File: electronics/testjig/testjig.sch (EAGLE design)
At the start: 13 parts, among them J3 ISP/DUT, Q1 12MHz, U1 MCP1824, U2 TINY84

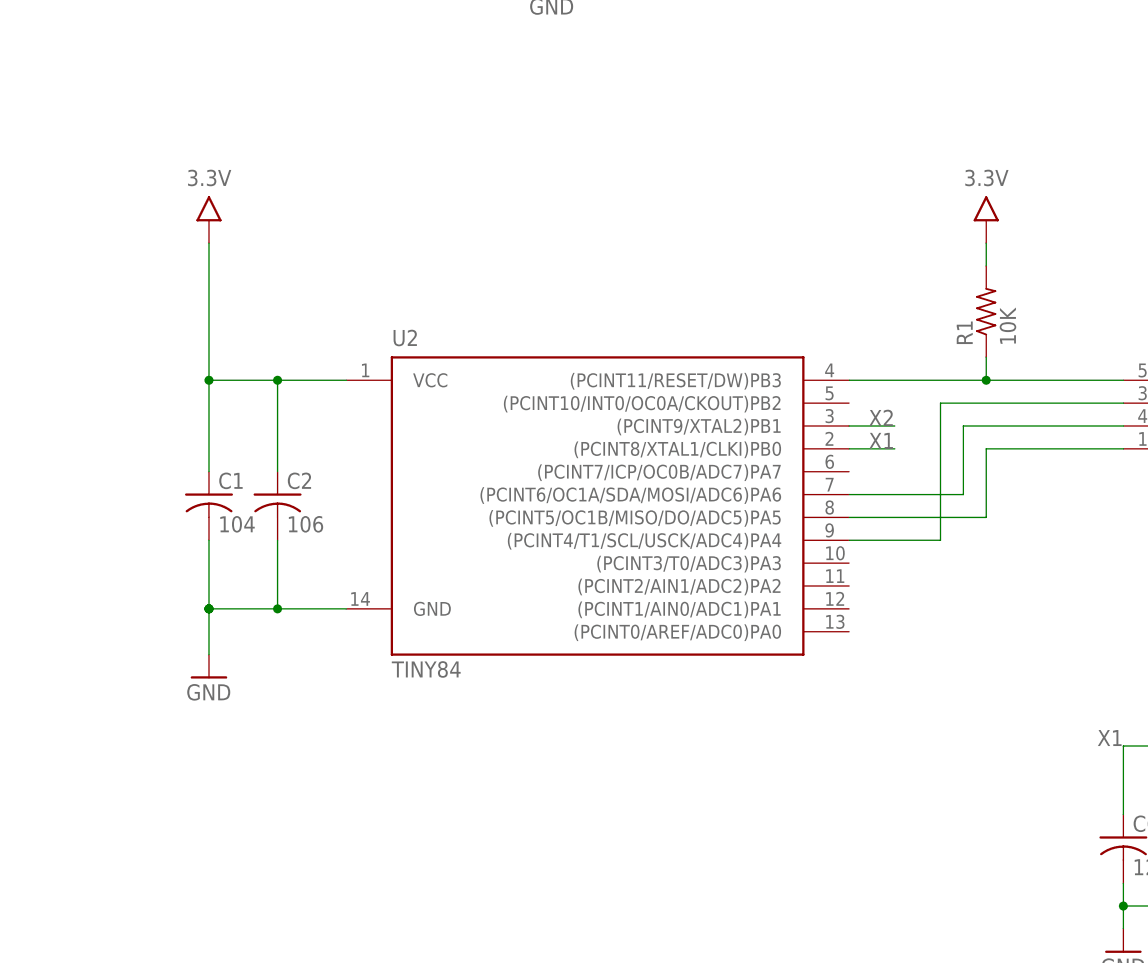
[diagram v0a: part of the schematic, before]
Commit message: Test jig initial(?)
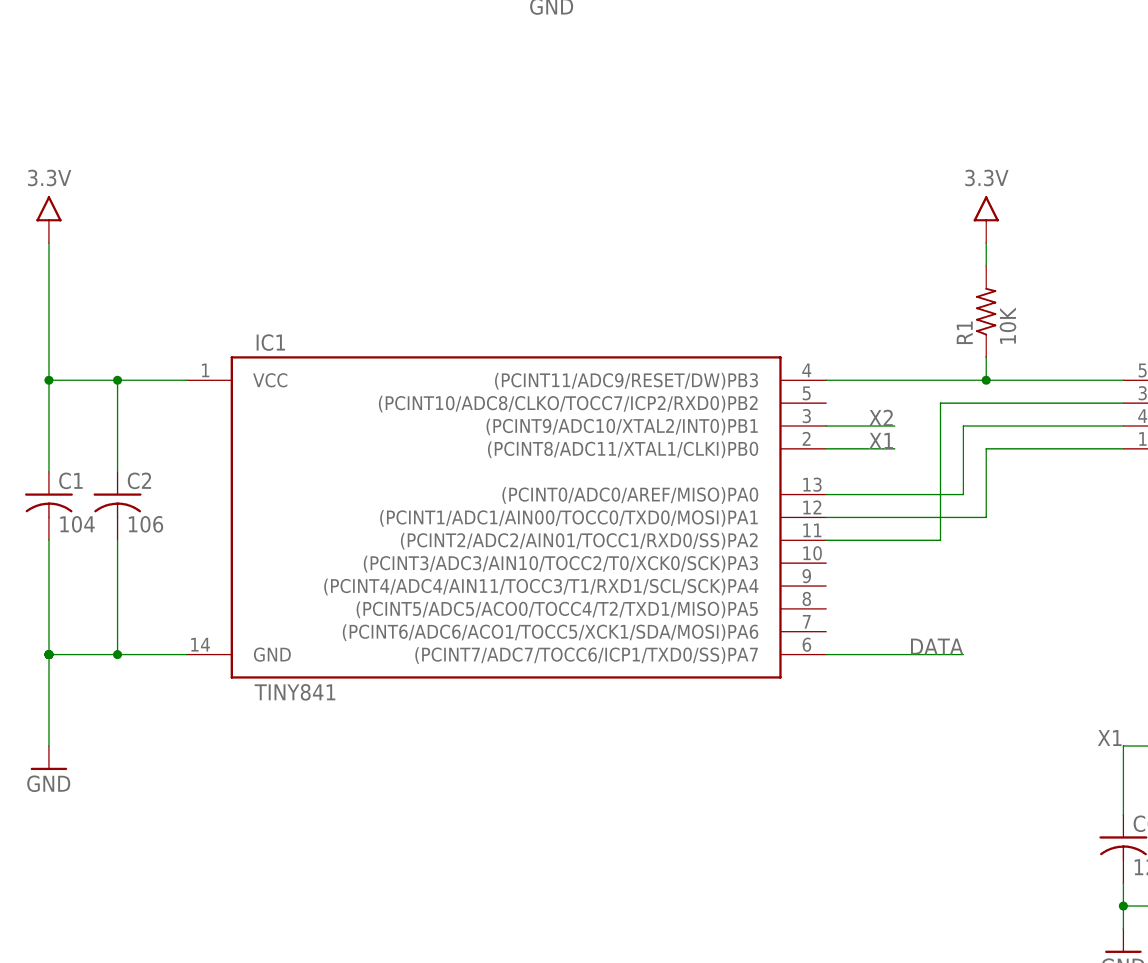
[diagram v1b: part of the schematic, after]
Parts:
- removed U2: TINY84, bt_avr:ATTINY24/44/84-SSU
- added IC1: TINY841, bt_avr:ATTINY441/841-SSU
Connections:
- removed net N$3: J3.MOSI, U2.(PCINT6/OC1A/SDA/MOSI/ADC6)PA6
- removed net N$4: J3.MISO, U2.(PCINT5/OC1B/MISO/DO/ADC5)PA5
- removed net N$5: J3.SCK, U2.(PCINT4/T1/SCL/USCK/ADC4)PA4
- new net PA0: IC1.(PCINT0/ADC0/AREF/MISO)PA0, J3.MOSI
- new net PA1: IC1.(PCINT1/ADC1/AIN00/TOCC0/TXD0/MOSI)PA1, J3.MISO
- new net PA2: IC1.(PCINT2/ADC2/AIN01/TOCC1/RXD0/SS)PA2, J3.SCK
- net 3.3V: now also IC1.VCC; no longer U2.VCC
- net DATA: now also IC1.(PCINT7/ADC7/TOCC6/ICP1/TXD0/SS)PA7
- net GND: now also IC1.GND; no longer U2.GND
- net RESET: now also IC1.(PCINT11/ADC9/RESET/DW)PB3; no longer U2.(PCINT11/RESET/DW)PB3
- net X1: now also IC1.(PCINT8/ADC11/XTAL1/CLKI)PB0; no longer U2.(PCINT8/XTAL1/CLKI)PB0
- net X2: now also IC1.(PCINT9/ADC10/XTAL2/INT0)PB1; no longer U2.(PCINT9/XTAL2)PB1
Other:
- moved on the sheet: C1, C2
